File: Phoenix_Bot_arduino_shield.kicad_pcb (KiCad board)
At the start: 2 copper layers, 102.9 x 54.6 mm, 0 parts

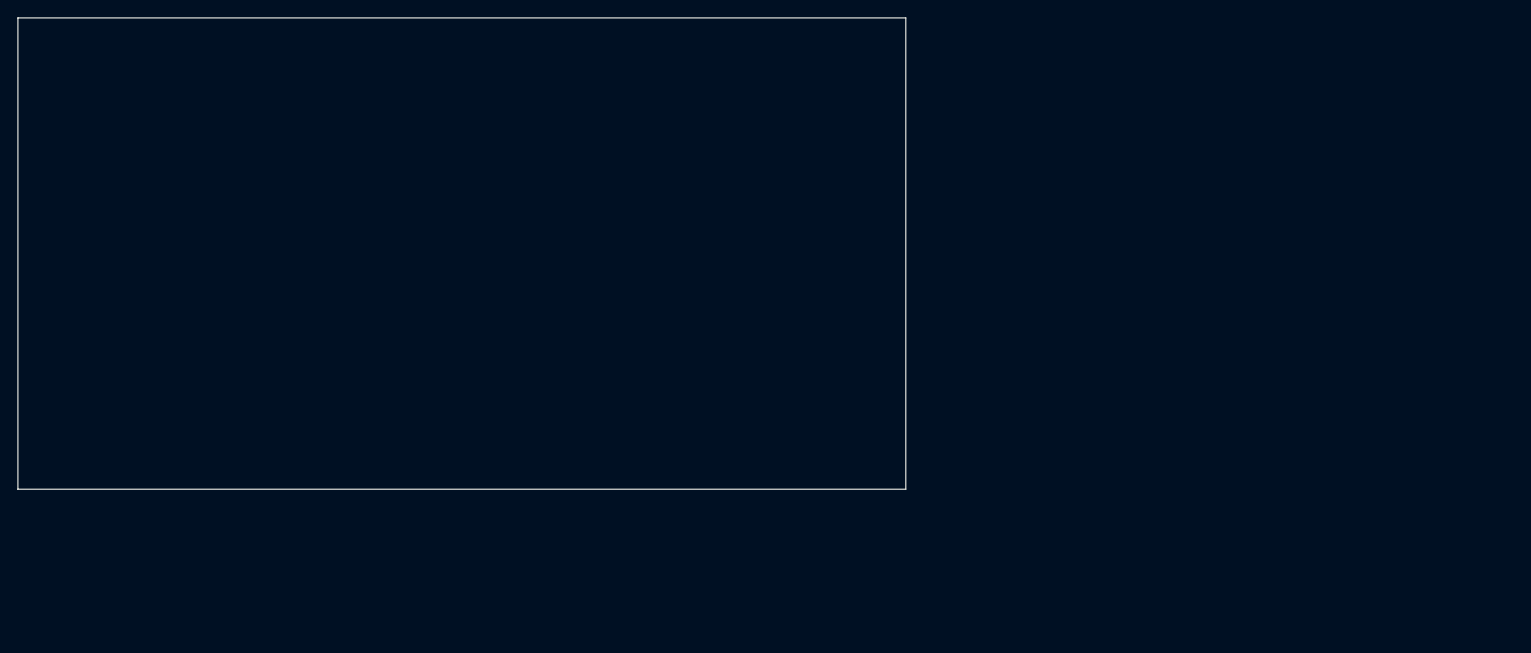
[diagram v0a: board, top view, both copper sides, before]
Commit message: Finished schematic and laid out PCB design
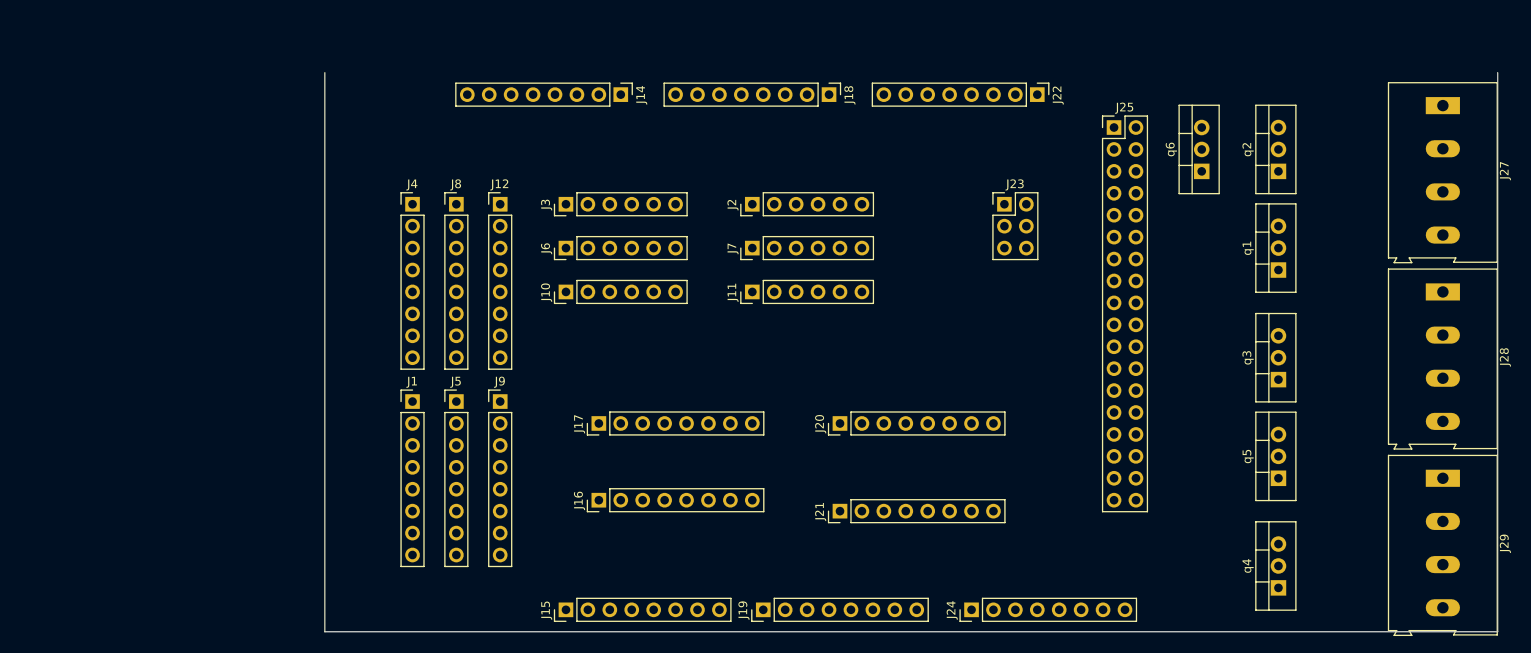
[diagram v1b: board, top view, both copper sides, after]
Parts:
- added J1: Analog_signal_male, Pin_Headers:Pin_Header_Straight_1x08_Pitch2.54mm, F.Cu at (121.9, 100.3)
- added J10: Ground, Pin_Headers:Pin_Header_Straight_1x06_Pitch2.54mm, F.Cu at (139.7, 87.6)
- added J11: Ground, Pin_Headers:Pin_Header_Straight_1x06_Pitch2.54mm, F.Cu at (161.3, 87.6)
- added J12: Ground, Pin_Headers:Pin_Header_Straight_1x08_Pitch2.54mm, F.Cu at (132.1, 77.5)
- added J14: PWN(10-5), Pin_Headers:Pin_Header_Straight_1x08_Pitch2.54mm, F.Cu at (146.1, 64.8)
- added J15: On Board Supply, Pin_Headers:Pin_Header_Straight_1x08_Pitch2.54mm, F.Cu at (139.7, 124.5)
- added J16: 1x8 Male, Pin_Headers:Pin_Header_Straight_1x08_Pitch2.54mm, F.Cu at (143.5, 111.8)
- added J17: 1x8 Male, Pin_Headers:Pin_Header_Straight_1x08_Pitch2.54mm, F.Cu at (143.5, 102.9)
- added J18: PWM_(6-1), Pin_Headers:Pin_Header_Straight_1x08_Pitch2.54mm, F.Cu at (170.2, 64.8)
- added J19: Analog_Pin_1, Pin_Headers:Pin_Header_Straight_1x08_Pitch2.54mm, F.Cu at (162.6, 124.5)
- added J2: Encoder_signal, Pin_Headers:Pin_Header_Straight_1x06_Pitch2.54mm, F.Cu at (161.3, 77.5)
- added J20: 1x8 Female, Pin_Headers:Pin_Header_Straight_1x08_Pitch2.54mm, F.Cu at (171.4, 102.9)
- added J21: 1x8 Female, Pin_Headers:Pin_Header_Straight_1x08_Pitch2.54mm, F.Cu at (171.4, 113.0)
- added J22: Serial, Pin_Headers:Pin_Header_Straight_1x08_Pitch2.54mm, F.Cu at (194.3, 64.8)
- added J23: ICSP, Pin_Headers:Pin_Header_Straight_2x03_Pitch2.54mm, F.Cu at (190.5, 77.5)
- added J24: Analog_Pin_2, Pin_Headers:Pin_Header_Straight_1x08_Pitch2.54mm, F.Cu at (186.7, 124.5)
- added J25: Digital_Pins, Pin_Headers:Pin_Header_Straight_2x18_Pitch2.54mm, F.Cu at (203.2, 68.6)
- added J27: Solenoid_terminal, Connectors_Terminal_Blocks:TerminalBlock_Altech_AK300-4_P5.00mm, F.Cu at (241.3, 66.0)
- added J28: Solendoid_middle_terminal, Connectors_Terminal_Blocks:TerminalBlock_Altech_AK300-4_P5.00mm, F.Cu at (241.3, 87.6)
- added J29: bottom_solenoid_terminal, Connectors_Terminal_Blocks:TerminalBlock_Altech_AK300-4_P5.00mm, F.Cu at (241.3, 109.2)
- added J3: Servo_signal, Pin_Headers:Pin_Header_Straight_1x06_Pitch2.54mm, F.Cu at (139.7, 77.5)
- added J4: Analog_signal_female, Pin_Headers:Pin_Header_Straight_1x08_Pitch2.54mm, F.Cu at (121.9, 77.5)
- added J5: Analog_signal_power, Pin_Headers:Pin_Header_Straight_1x08_Pitch2.54mm, F.Cu at (127.0, 100.3)
- added J6: Servo_Power, Pin_Headers:Pin_Header_Straight_1x06_Pitch2.54mm, F.Cu at (139.7, 82.5)
- added J7: Encoder_Power, Pin_Headers:Pin_Header_Straight_1x06_Pitch2.54mm, F.Cu at (161.3, 82.5)
- added J8: Analog_Power_female, Pin_Headers:Pin_Header_Straight_1x08_Pitch2.54mm, F.Cu at (127.0, 77.5)
- added J9: Ground, Pin_Headers:Pin_Header_Straight_1x08_Pitch2.54mm, F.Cu at (132.1, 100.3)
- added q1: solenoid_1, TO_SOT_Packages_THT:TO-220-3_Vertical, F.Cu at (222.2, 85.1)
- added q2: solenoid_4, TO_SOT_Packages_THT:TO-220-3_Vertical, F.Cu at (222.2, 73.7)
- added q3: solenoid_3, TO_SOT_Packages_THT:TO-220-3_Vertical, F.Cu at (222.2, 97.8)
- added q4: solenoid_5, TO_SOT_Packages_THT:TO-220-3_Vertical, F.Cu at (222.2, 121.9)
- added q5: solenoid_3, TO_SOT_Packages_THT:TO-220-3_Vertical, F.Cu at (222.2, 109.2)
- added q6: solenoid_6, TO_SOT_Packages_THT:TO-220-3_Vertical, F.Cu at (213.4, 73.7)
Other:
- board size 102.9 x 54.6 mm -> 135.9 x 64.8 mm
